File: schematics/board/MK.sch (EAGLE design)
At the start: 56 parts

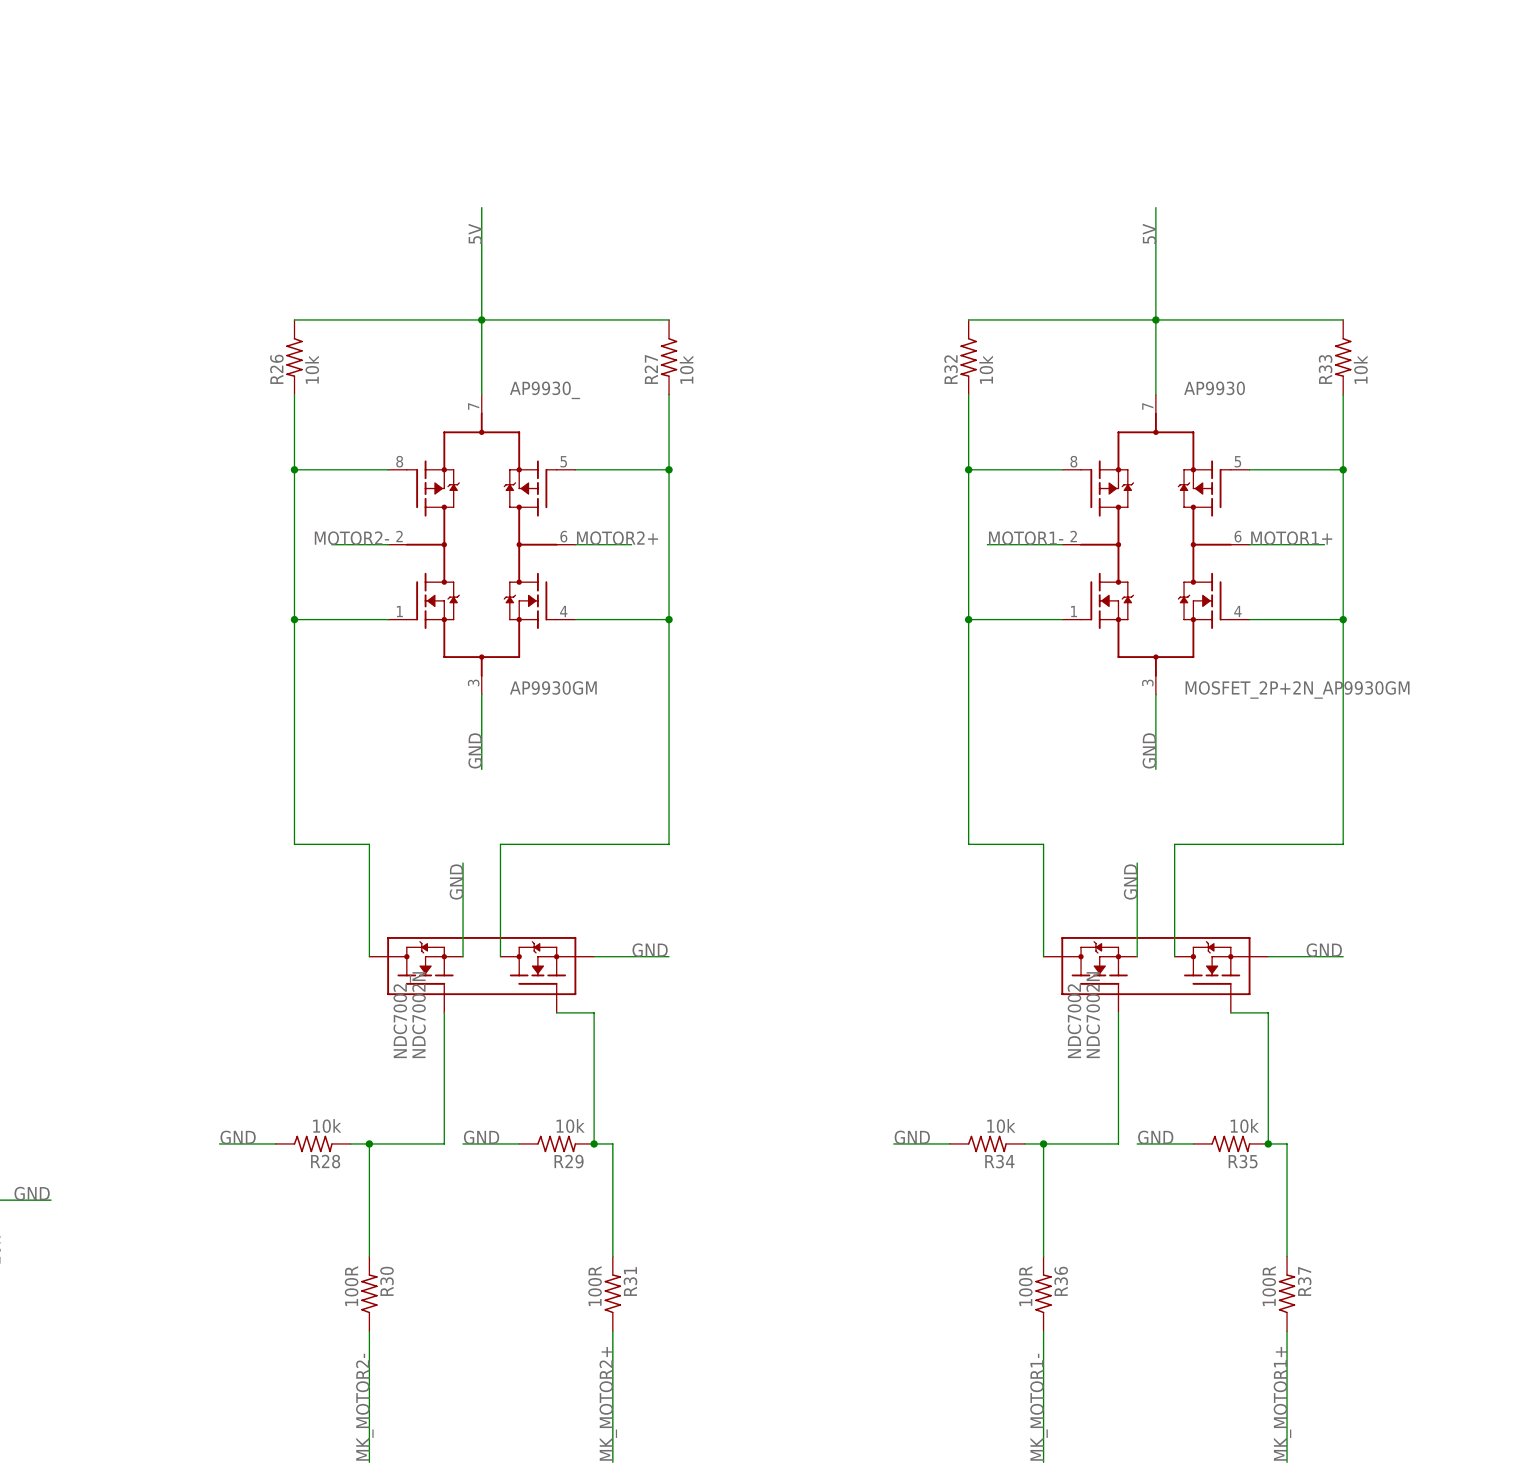
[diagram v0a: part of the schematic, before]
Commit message: СД в центре лепестка. Платы версия 2
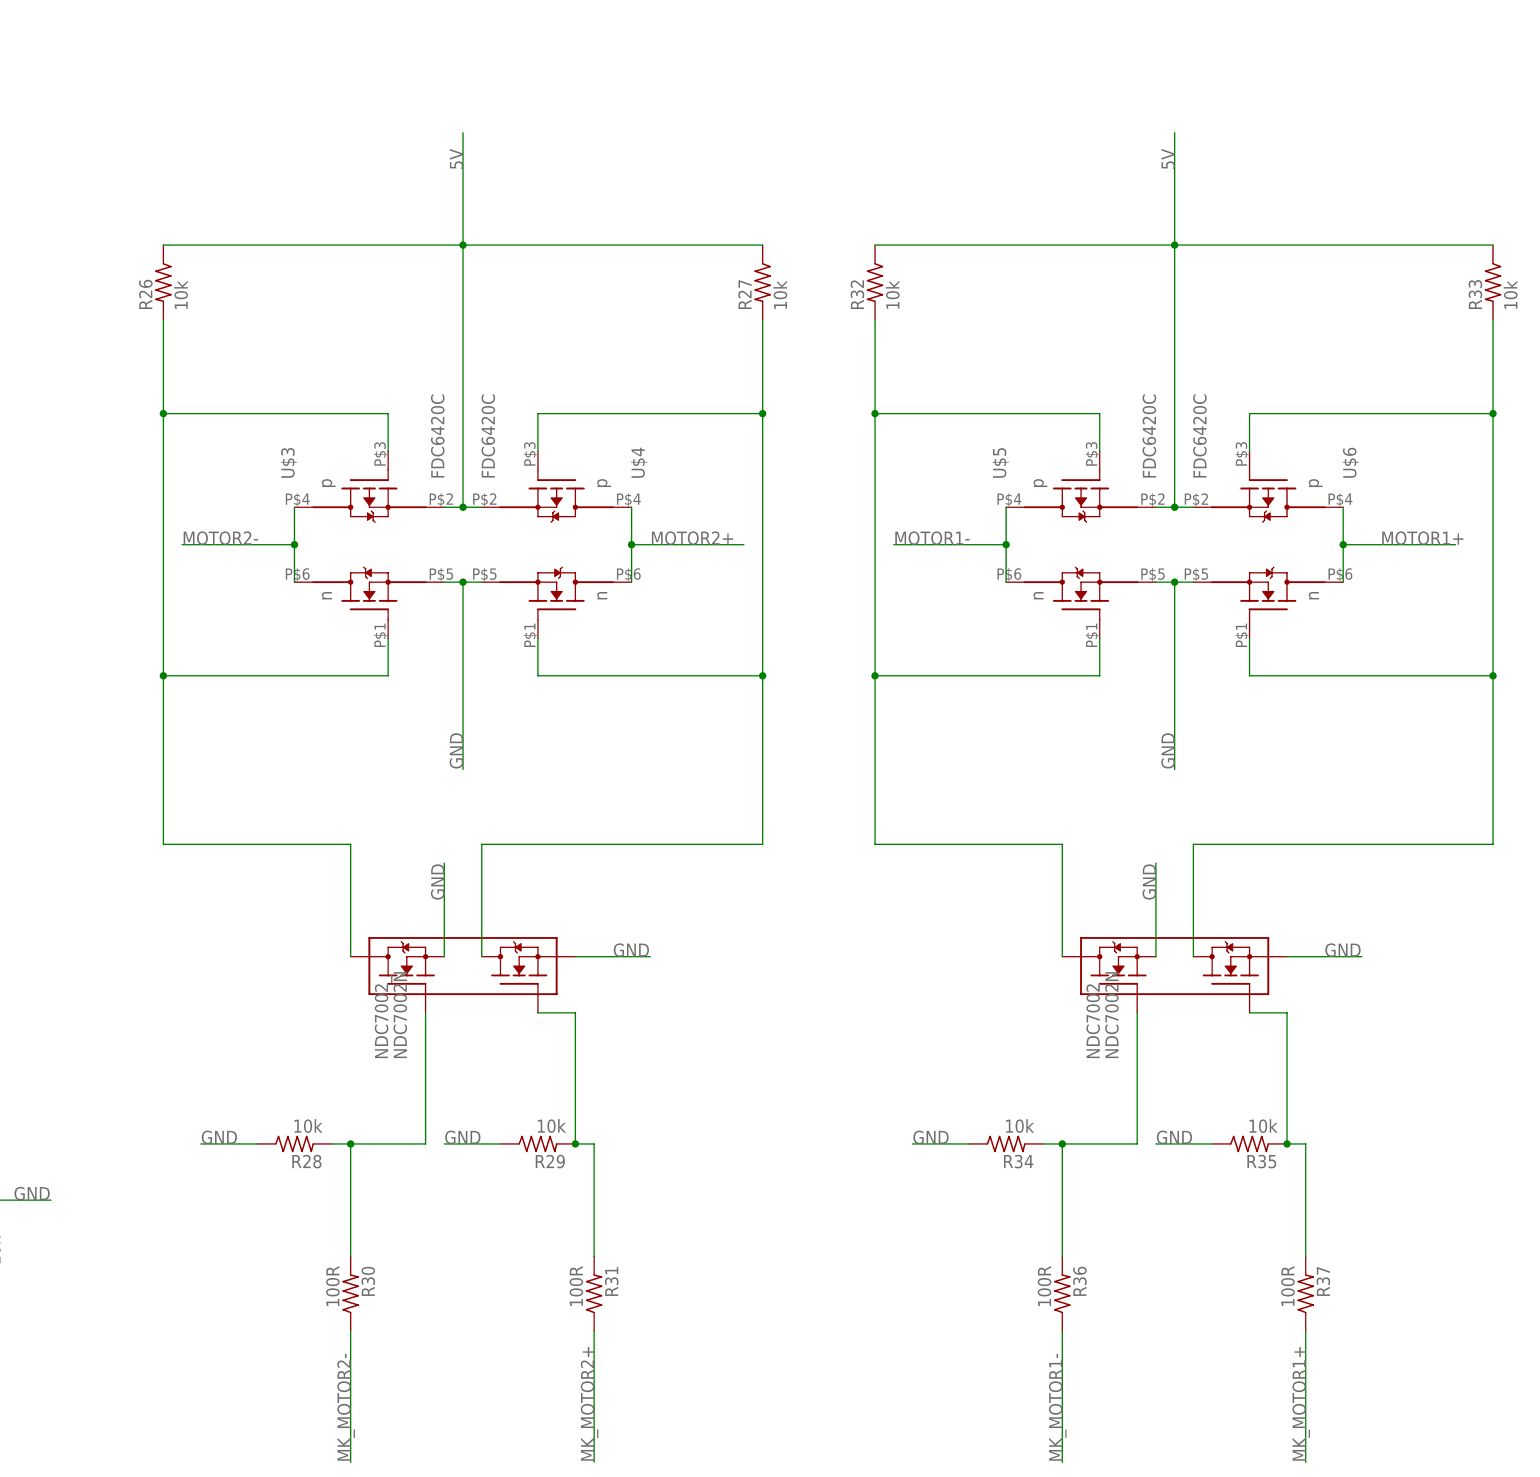
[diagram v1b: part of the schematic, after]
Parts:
- removed AP9930: MOSFET_2P+2N_AP9930GM, UNKNOWN-2024:MOSFET_2P+2N_AP9930GM
- removed AP9930_: AP9930GM, UNKNOWN-2024:MOSFET_2P+2N_AP9930GM
- added U$3, U$4, U$5, U$6: FDC6420C, KNPN-2023:FDC6420C
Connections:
- net 5V: now also U$3.PS, U$4.PS, U$5.PS, U$6.PS; no longer AP9930.P1P2S, AP9930_.P1P2S
- net GND: now also U$3.NS, U$4.NS, U$5.NS, U$6.NS; no longer AP9930.N1N2S, AP9930_.N1N2S
- net MOTOR1+: now also U$6.ND, U$6.PD; no longer AP9930.P2N2D
- net MOTOR1-: now also U$5.ND, U$5.PD; no longer AP9930.P1N1D
- net MOTOR2+: now also U$4.ND, U$4.PD; no longer AP9930_.P2N2D
- net MOTOR2-: now also U$3.ND, U$3.PD; no longer AP9930_.P1N1D
- net N$24: now also U$5.NG, U$5.PG; no longer AP9930.N1G, AP9930.P1G
- net N$25: now also U$3.NG, U$3.PG; no longer AP9930_.N1G, AP9930_.P1G
- net N$26: now also U$4.NG, U$4.PG; no longer AP9930_.N2G, AP9930_.P2G
- net N$27: now also U$6.NG, U$6.PG; no longer AP9930.N2G, AP9930.P2G
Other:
- moved on the sheet: NDC7002, NDC7002_, R26, R27, R28, R29, R30, R31, R32, R33, R34, R35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
